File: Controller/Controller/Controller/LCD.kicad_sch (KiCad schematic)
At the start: 46 parts, among them J8 Conn_01x06_MountingPin, J9 Conn_01x50_MountingPin, Q1 CSD16323Q3, U10 LTC1261L, U4 LM317_TO-252, U5 AMS1117-3.3, U6 LM317_TO-252, U7 LM3488, U8 C85037, U9 LM317_TO-252

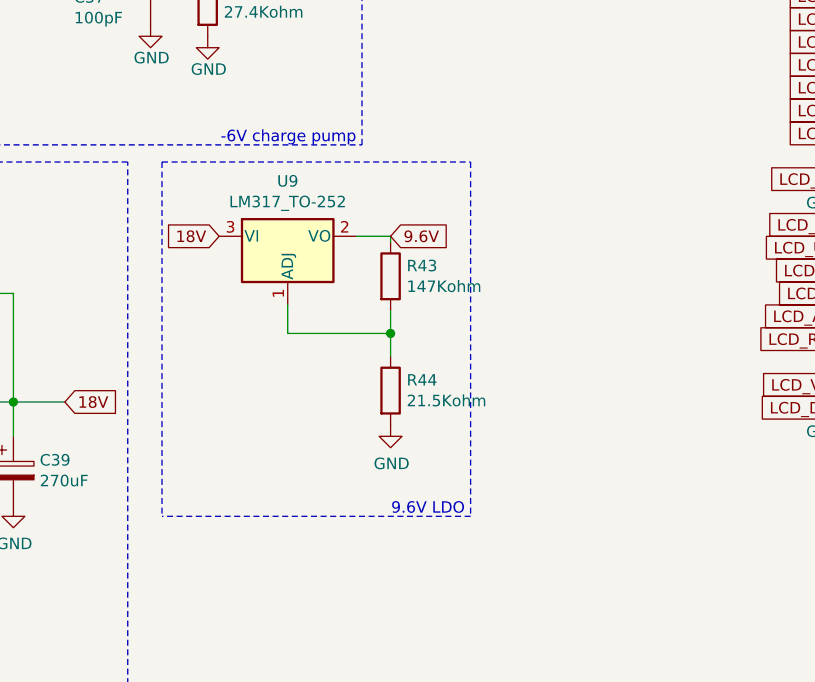
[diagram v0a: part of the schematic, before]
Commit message: contoller and contoller front Rev 1
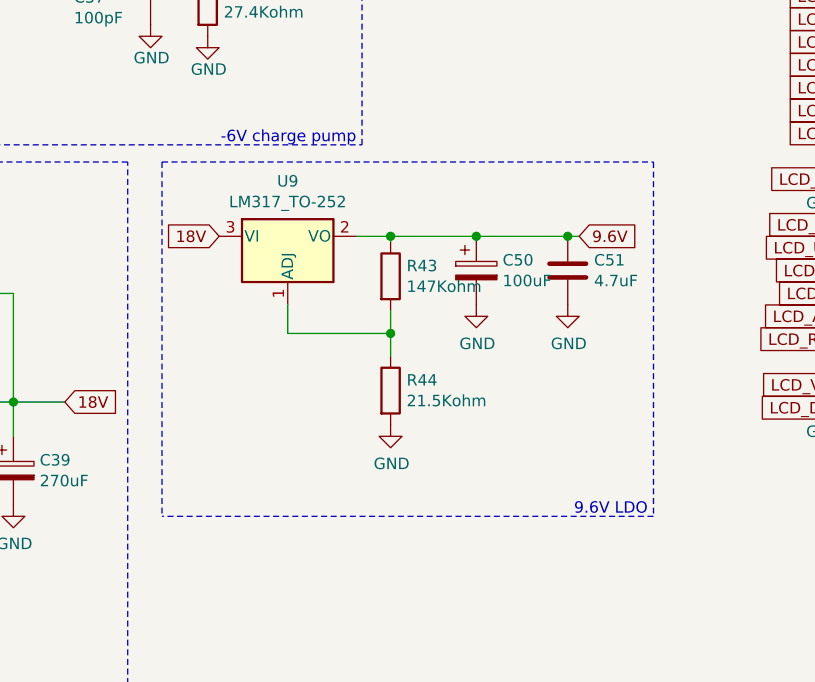
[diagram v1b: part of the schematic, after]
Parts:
- added C50: 100uF, Capacitor_SMD:CP_Elec_5x5.4, symbol Device:CP
- added C51: 4.7uF, Capacitor_SMD:C_0805_2012Metric_Pad1.18x1.45mm_HandSolder, symbol Device:C
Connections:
- net 9.6V: now also C50.1, C51.1
- net GND: now also C50.2, C51.2
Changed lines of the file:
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@@
   (junction (at 179.07 79.375) (diameter 1.016) (color 0 0 0 0))
   (junction (at 179.07 86.995) (diameter 1.016) (color 0 0 0 0))
+  (junction (at 199.39 118.11) (diameter 1.016) (color 0 0 0 0))
   (junction (at 199.39 128.905) (diameter 1.016) (color 0 0 0 0))
+  (junction (at 208.915 118.11) (diameter 1.016) (color 0 0 0 0))
+  (junction (at 219.075 118.11) (diameter 1.016) (color 0 0 0 0))
   (junction (at 257.81 20.32) (diameter 1.016) (color 0 0 0 0))
   (junction (at 257.81 25.4) (diameter 1.016) (color 0 0 0 0))
@@
     (stroke (width 0) (type solid) (color 0 0 0 0))
   )
+  (wire (pts (xy 199.39 118.11) (xy 208.915 118.11))
+    (stroke (width 0) (type solid) (color 0 0 0 0))
+  )
   (wire (pts (xy 199.39 118.745) (xy 199.39 118.11))
     (stroke (width 0) (type solid) (color 0 0 0 0))
@@
     (stroke (width 0) (type solid) (color 0 0 0 0))
   )
+  (wire (pts (xy 208.915 118.11) (xy 219.075 118.11))
+    (stroke (width 0) (type solid) (color 0 0 0 0))
+  )
+  (wire (pts (xy 219.075 118.11) (xy 220.345 118.11))
+    (stroke (width 0) (type solid) (color 0 0 0 0))
+  )
   (wire (pts (xy 252.73 48.26) (xy 257.81 48.26))
     (stroke (width 0) (type solid) (color 0 0 0 0))
@@
     (stroke (width 0) (type dash) (color 0 0 0 0))
   )
-  (polyline (pts (xy 173.99 109.855) (xy 208.28 109.855))
+  (polyline (pts (xy 173.99 109.855) (xy 228.6 109.855))
     (stroke (width 0) (type dash) (color 0 0 0 0))
   )
@@
     (stroke (width 0) (type dash) (color 0 0 0 0))
   )
-  (polyline (pts (xy 208.28 109.855) (xy 208.28 149.225))
-    (stroke (width 0) (type dash) (color 0 0 0 0))
-  )
-  (polyline (pts (xy 208.28 149.225) (xy 173.99 149.225))
+  (polyline (pts (xy 228.6 109.855) (xy 228.6 149.225))
+    (stroke (width 0) (type dash) (color 0 0 0 0))
+  )
+  (polyline (pts (xy 228.6 149.225) (xy 173.99 149.225))
     (stroke (width 0) (type dash) (color 0 0 0 0))
   )
@@
     (effects (font (size 1.27 1.27)) (justify right bottom))
   )
-  (text "9.6V LDO\n" (at 207.645 149.225 180)
+  (text "9.6V LDO\n" (at 227.965 149.225 180)
     (effects (font (size 1.27 1.27)) (justify right bottom))
   )
@@
     )
   )
-  (global_label "9.6V" (shape input) (at 199.39 118.11 0)
-    (effects (font (size 1.27 1.27)) (justify left))
-    (property "Intersheet References" "${INTERSHEET_REFS}" (id 0) (at 207.4395 118.0306 0)
-      (effects (font (size 1.27 1.27)) (justify left) hide)
-    )
-  )
   (global_label "9.6V" (shape input) (at 203.2 22.86 0)
     (effects (font (size 1.27 1.27)) (justify left))
@@
     )
   )
+  (global_label "9.6V" (shape input) (at 220.345 118.11 0)
+    (effects (font (size 1.27 1.27)) (justify left))
+    (property "Intersheet References" "${INTERSHEET_REFS}" (id 0) (at 228.3945 118.0306 0)
+      (effects (font (size 1.27 1.27)) (justify left) hide)
+    )
+  )
   (global_label "LCD_B7" (shape input) (at 252.73 48.26 180)
     (effects (font (size 1.27 1.27)) (justify right))
@@
     (pin "1")
   )
+  (symbol (lib_id "power:GND") (at 208.915 125.73 0) (unit 1)
+    (in_bom yes) (on_board yes)
+    (property "Reference" "#PWR0143" (id 0) (at 208.915 132.08 0)
+      (effects (font (size 1.27 1.27)) hide)
+    )
+    (property "Value" "GND" (id 1) (at 209.0293 130.0544 0))
+    (property "Footprint" "" (id 2) (at 208.915 125.73 0)
+      (effects (font (size 1.27 1.27)) hide)
+    )
+    (property "Datasheet" "" (id 3) (at 208.915 125.73 0)
+      (effects (font (size 1.27 1.27)) hide)
+    )
+    (pin "1")
+  )
+  (symbol (lib_id "power:GND") (at 219.075 125.73 0) (unit 1)
+    (in_bom yes) (on_board yes)
+    (property "Reference" "#PWR0142" (id 0) (at 219.075 132.08 0)
+      (effects (font (size 1.27 1.27)) hide)
+    )
+    (property "Value" "GND" (id 1) (at 219.1893 130.0544 0))
+    (property "Footprint" "" (id 2) (at 219.075 125.73 0)
+      (effects (font (size 1.27 1.27)) hide)
+    )
+    (property "Datasheet" "" (id 3) (at 219.075 125.73 0)
+      (effects (font (size 1.27 1.27)) hide)
+    )
+    (pin "1")
+  )
   (symbol (lib_id "power:GND") (at 252.73 109.22 270) (unit 1)
     (in_bom yes) (on_board yes)
@@
       (effects (font (size 1.27 1.27)) hide)
     )
+    (pin "1")
+    (pin "2")
+  )
+  (symbol (lib_id "Device:CP") (at 208.915 121.92 0) (unit 1)
+    (in_bom yes) (on_board yes)
+    (property "Reference" "C50" (id 0) (at 211.8361 120.7706 0)
+      (effects (font (size 1.27 1.27)) (justify left))
+    )
+    (property "Value" "100uF" (id 1) (at 211.836 123.069 0)
+      (effects (font (size 1.27 1.27)) (justify left))
+    )
+    (property "Footprint" "Capacitor_SMD:CP_Elec_5x5.4" (id 2) (at 209.8802 125.73 0)
+      (effects (font (size 1.27 1.27)) hide)
+    )
+    (property "Datasheet" "~" (id 3) (at 208.915 121.92 0)
+      (effects (font (size 1.27 1.27)) hide)
+    )
+    (pin "1")
+    (pin "2")
+  )
+  (symbol (lib_id "Device:C") (at 219.075 121.92 0) (unit 1)
+    (in_bom yes) (on_board yes)
+    (property "Reference" "C51" (id 0) (at 221.9961 120.7706 0)
+      (effects (font (size 1.27 1.27)) (justify left))
+    )
+    (property "Value" "4.7uF" (id 1) (at 221.9961 123.0693 0)
+      (effects (font (size 1.27 1.27)) (justify left))
+    )
+    (property "Footprint" "Capacitor_SMD:C_0805_2012Metric_Pad1.18x1.45mm_HandSolder" (id 2) (at 220.0402 125.73 0)
+      (effects (font (size 1.27 1.27)) hide)
+    )
+    (property "Datasheet" "~" (id 3) (at 219.075 121.92 0)
+      (effects (font (size 1.27 1.27)) hide)
+    )
+    (property "LCSC" "C415307" (id 4) (at 219.075 121.92 0)
+      (effects (font (size 1.27 1.27)) hide)
+    )

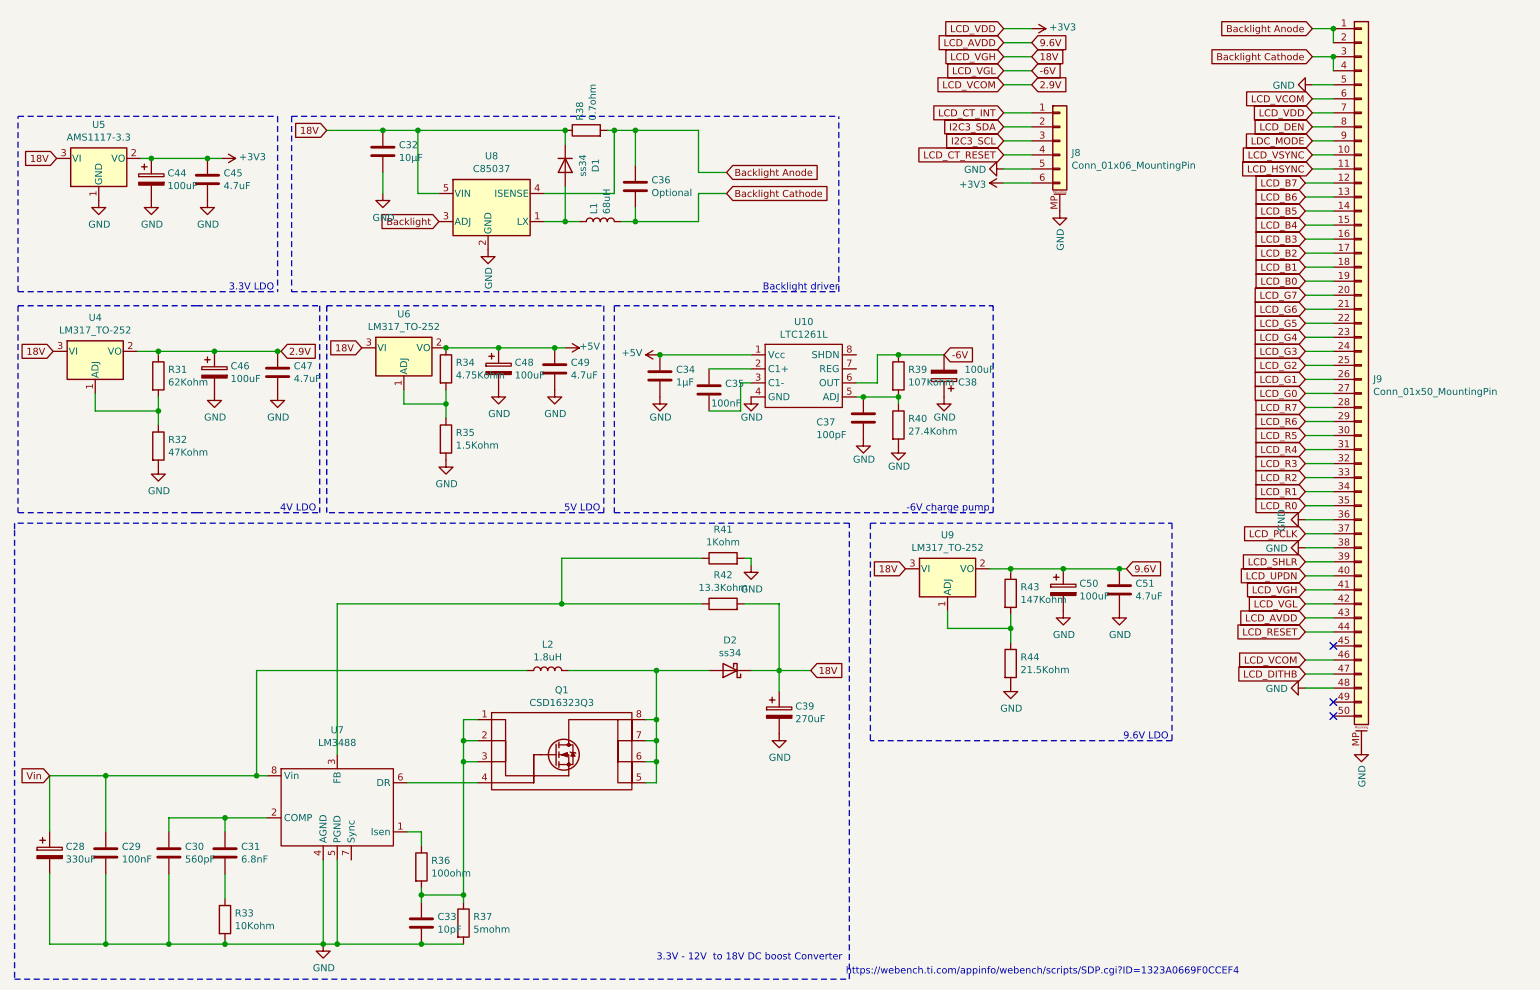
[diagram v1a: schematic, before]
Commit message: Rev 3 Pcb's
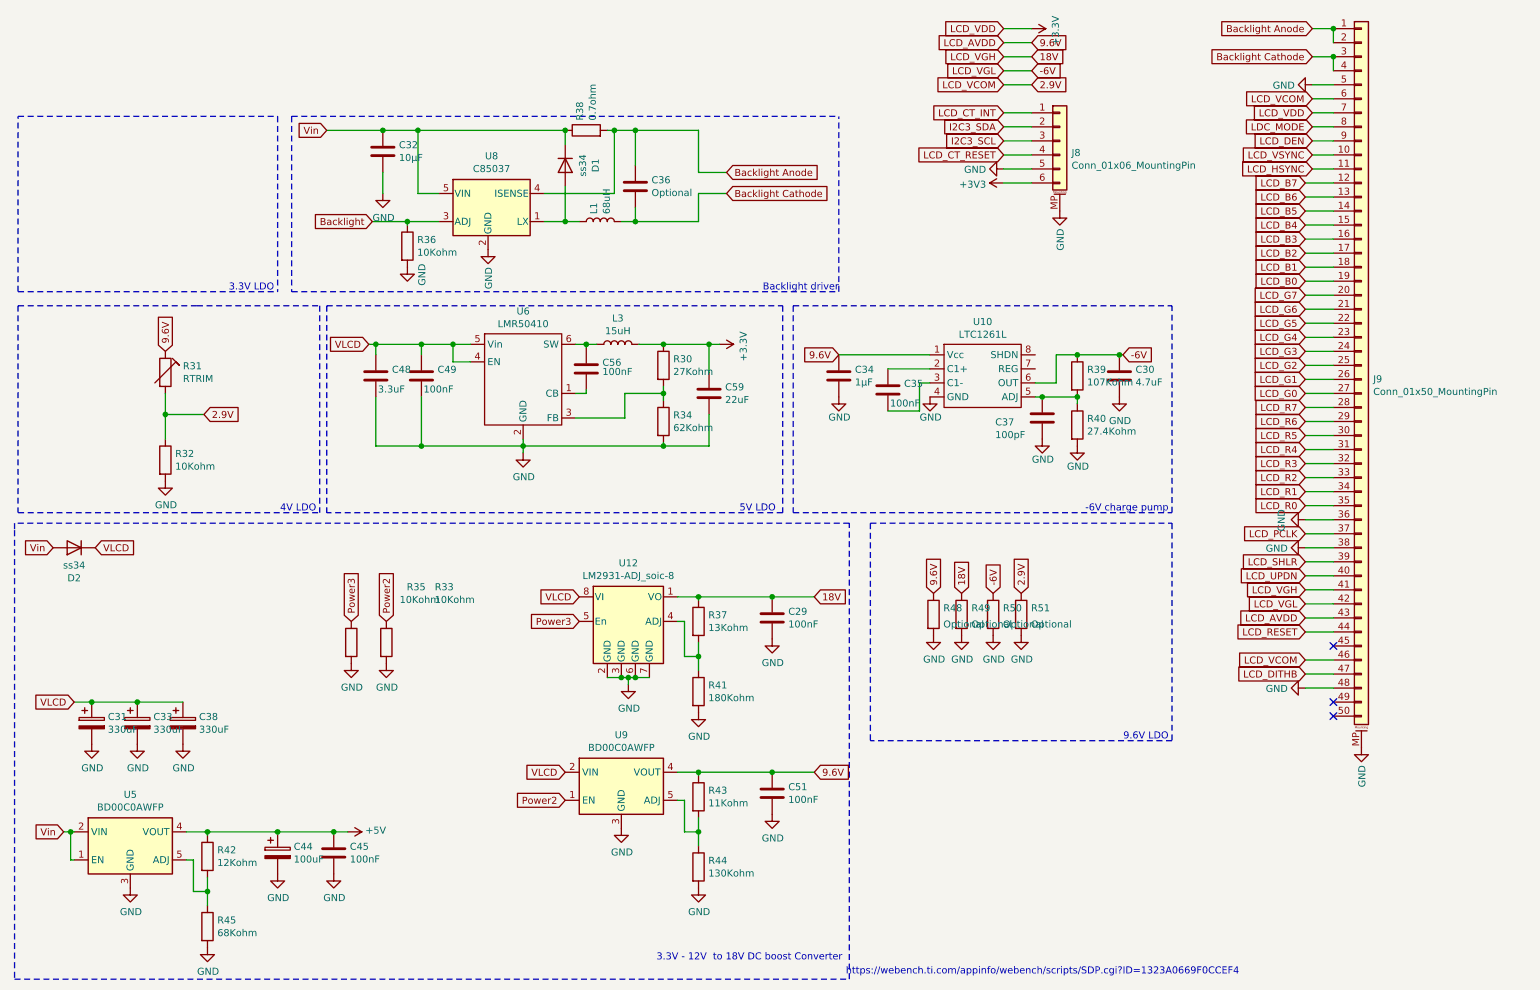
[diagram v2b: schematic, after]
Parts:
- removed C28: 330uF, Capacitor_SMD:CP_Elec_8x10, symbol Device:CP
- removed C31: 6.8nF, Capacitor_SMD:C_0805_2012Metric_Pad1.18x1.45mm_HandSolder, symbol Device:C
- removed C33: 10pF, Capacitor_SMD:C_0805_2012Metric_Pad1.18x1.45mm_HandSolder, symbol Device:C
- removed C39: 270uF, Capacitor_SMD:CP_Elec_10x12.6, symbol Device:CP
- removed C46, C48, C50: 100uF, Capacitor_SMD:CP_Elec_5x5.4, symbol Device:CP
- removed C47: 4.7uF, Capacitor_SMD:C_0805_2012Metric_Pad1.18x1.45mm_HandSolder, symbol Device:C
- removed D2: ss34, Diode_SMD:D_SMA_Handsoldering, symbol Device:D_Schottky
- removed L2: 1.8uH, Inductor_SMD:L_6.3x6.3_H3, symbol Device:L
- removed Q1: CSD16323Q3, Package_TO_SOT_SMD:TDSON-8-1, symbol 01-Global-LIB:CSD16323Q3
- removed R31: 62Kohm, Resistor_SMD:R_0805_2012Metric_Pad1.20x1.40mm_HandSolder, symbol Device:R
- removed U4, U6, U9: LM317_TO-252, Package_TO_SOT_SMD:TO-252-2, symbol Regulator_Linear:LM317_TO-252
- removed U5: AMS1117-3.3, Package_TO_SOT_SMD:SOT-223-3_TabPin2, symbol Regulator_Linear:AMS1117-3.3
- removed U7: LM3488, Package_SO:MSOP-8_3x3mm_P0.65mm, symbol 01-Global-LIB:LM3488
- added C31, C33: 330uF, Capacitor_SMD:CP_Elec_10x10.5, symbol Device:CP
- added C48: 3.3uF, Capacitor_SMD:CP_Elec_4x5.7, symbol Device:C
- added C56: 100nF, Capacitor_SMD:C_0805_2012Metric_Pad1.18x1.45mm_HandSolder, symbol Device:C
- added C59: 22uF, Capacitor_SMD:CP_Elec_3x5.3, symbol Device:C
- added D2: ss34, Diode_SMD:D_SMA_Handsoldering, symbol Device:D
- added L3: 15uH, Inductor_SMD:L_10.4x10.4_H4.8, symbol Device:L
- added R30: 27Kohm, Resistor_SMD:R_0805_2012Metric_Pad1.20x1.40mm_HandSolder, symbol Device:R
- added R31: RTRIM, Potentiometer_SMD:Potentiometer_Bourns_3214J_Horizontal, symbol Device:RTRIM
- added R45: 68Kohm, Resistor_SMD:R_0805_2012Metric_Pad1.20x1.40mm_HandSolder, symbol Device:R
- added R48, R49, R50, R51: Optional, Resistor_SMD:R_0805_2012Metric_Pad1.20x1.40mm_HandSolder, symbol Device:R
- added U12: LM2931-ADJ_soic-8, Package_SO:SOIC-8_3.9x4.9mm_P1.27mm, symbol 00_LIB:LM2931-ADJ_soic-8
- added U5, U9: BD00C0AWFP, Package_TO_SOT_SMD:TO-252-5_TabPin3, symbol Regulator_Linear:MIC29152WU
- added U6: LMR50410, Package_TO_SOT_SMD:TSOT-23-6_HandSoldering, symbol 00_LIB:LMR50410
- C29: LCSC (none) -> C168908; Orderd (none) -> 100
- C30: value 560pF -> 4.7uF; LCSC C1829 -> C168908; Orderd (none) -> 100
- C32: LCSC C17024 -> C14860; Orderd (none) -> 10
- C34, C37: Orderd (none) -> 200
- C35: Orderd (none) -> 1000
- C38: value 100uF -> 330uF; footprint Capacitor_SMD:CP_Elec_5x5.4 -> Capacitor_SMD:CP_Elec_10x10.5; LCSC (none) -> C19606; Orderd (none) -> 20
- C45, C51: value 4.7uF -> 100nF; LCSC C415307 -> C168908; Orderd (none) -> 100
- C49: value 4.7uF -> 100nF; LCSC C415307 -> (none); Orderd (none) -> 1000
- D1, R38, R39, R40: Orderd (none) -> 100
- J8, J9: Orderd (none) -> 10
- R32: value 47Kohm -> 10Kohm
- R34: value 4.75Kohm -> 62Kohm; LCSC C706245 -> C422851; Orderd (none) -> 100
- R35: value 1.5Kohm -> 10Kohm; LCSC C203762 -> (none)
- R36: value 100ohm -> 10Kohm
- R37: value 5mohm -> 13Kohm; footprint Resistor_SMD:R_2512_6332Metric_Pad1.40x3.35mm_HandSolder -> Resistor_SMD:R_0805_2012Metric_Pad1.20x1.40mm_HandSolder; LCSC C782251 -> C170031
- R41: value 1Kohm -> 180Kohm; LCSC (none) -> C706267
- R42: value 13.3Kohm -> 12Kohm; LCSC C103975 -> C170031
- R43: value 147Kohm -> 11Kohm
- R44: value 21.5Kohm -> 130Kohm
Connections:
- net +3V3: now also C59.1, L3.2, R30.1; no longer C44.1, C45.1
- net +5V: now also C44.1, C45.1, R42.1, U5.4 (VOUT); no longer C34.1, C49.1, R34.1, U10.1 (Vcc)
- net -6V: now also C30.1, R50.1; no longer C38.2
- net 18V: now also C29.1, R37.1, R49.1, U12.1 (VO); no longer C32.1, D1.1 (K), R38.1, R42.2, U8.5 (VIN)
- net 2.9V: now also R32.1, R31.2, R51.1
- net 9.6V: now also C34.1, U10.1 (Vcc), R31.1, R48.1, U9.4 (VOUT)
- net Backlight: now also R36.1
- net GND: now also C38.2, R34.2, R36.2, C31.2, C33.2, C48.2, C59.2, R45.2, R48.2, R49.2, R50.2, R51.2, U12.2 (GND), U12.3 (GND), U12.6 (GND), U12.7 (GND), U5.3 (GND), U6.2 (GND), U9.3 (GND); no longer C38.1, R37.2
- net LCD_DEN: now also J9.9 (Pin_9); no longer J9.8 (Pin_8)
- net LDC_MODE: now also J9.8 (Pin_8); no longer J9.9 (Pin_9)
- net Vin: now also C32.1, D1.1 (K), R38.1, U8.5 (VIN), D2.2 (A), U5.1 (EN), U5.2 (VIN); no longer C29.1
- net Power2: now reaches R33.1
- net Power2: now also U9.1 (EN)
- net at R41.1: now also R37.2, U12.4 (ADJ); no longer R42.1
- net at R43.2, R44.1: now also U9.5 (ADJ)
- net Power3: now reaches R35.1
- net Power3: now also U12.5 (En); no longer R34.2
- new net: R42.2, R45.1, U5.5 (ADJ)
- new net: R30.2, R34.1, U6.3 (FB)
- new net: C56.1, L3.1, U6.6 (SW)
- new net: C56.2, U6.1 (CB)
- new net VLCD: C31.1, C33.1, C38.1, C48.1, C49.1, D2.1 (K), U12.8 (VI), U6.4 (EN), U6.5 (Vin), U9.2 (VIN)
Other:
- moved on the sheet: C34, C35, C37, C44, C45, C51, R39, R40, R43, R44, U10
